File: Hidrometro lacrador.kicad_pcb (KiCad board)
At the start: 2 copper layers, 4 parts, among them U1 ESP32-WROOM-V1

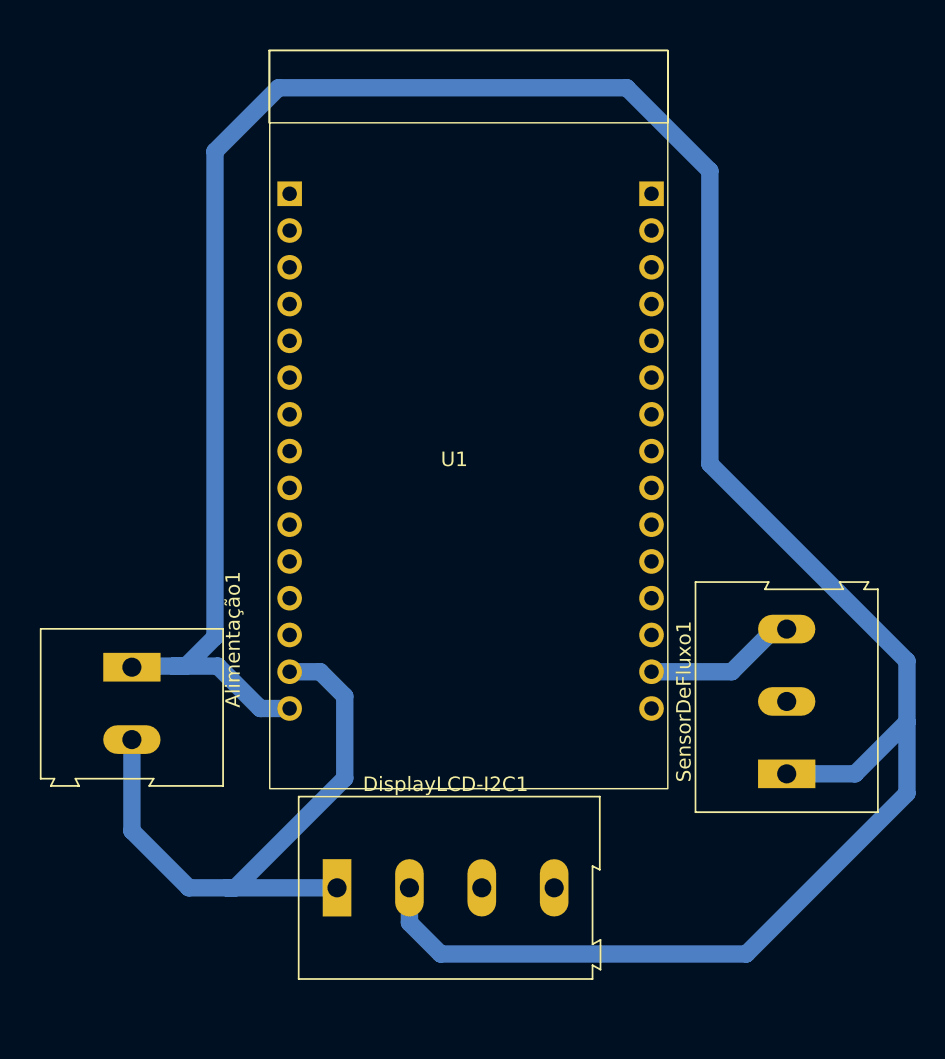
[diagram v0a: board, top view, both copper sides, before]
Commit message: Finalização do circuito e da PCB
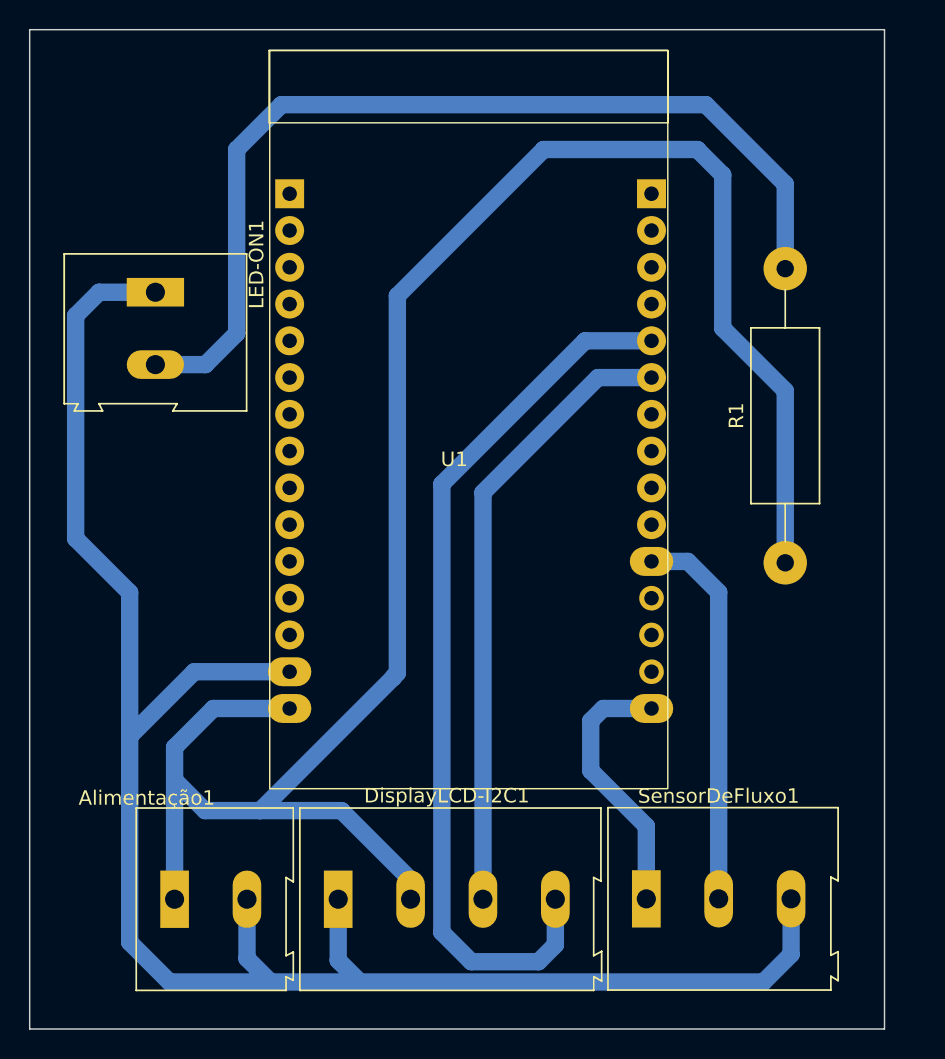
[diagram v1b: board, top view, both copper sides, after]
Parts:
- added LED-ON1: LED, TerminalBlock:TerminalBlock_Altech_AK300-2_P5.00mm, F.Cu at (31.1, 42.4)
- added R1: 330, Resistor_THT:R_Axial_DIN0414_L11.9mm_D4.5mm_P20.32mm_Horizontal, F.Cu at (74.6, 61.1)
- moved Alimentação1 16.3 mm to (32.4, 84.4), turned to 0 degrees
- moved SensorDeFluxo1 13.0 mm to (65.0, 84.3), turned to 0 degrees
- moved DisplayLCD-I2C1 0.79 mm to (43.7, 84.4)
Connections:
- DisplayLCD-I2C1 pad 3: unconnected-(DisplayLCD-I2C1-Pin_3-Pad3) -> I2C_SDA
- DisplayLCD-I2C1 pad 4: unconnected-(DisplayLCD-I2C1-Pin_4-Pad4) -> I2C_SCL
- SensorDeFluxo1 pad 1: +5V -> +3.3V
- SensorDeFluxo1 pad 2: unconnected-(SensorDeFluxo1-Pin_2-Pad2) -> GPIO-04
- U1 pad 20: unconnected-(U1-GPI21/I2C_SDA-Pad20) -> I2C_SCL
- U1 pad 21: unconnected-(U1-GPI19/VSPI_MISO-Pad21) -> I2C_SDA
- U1 pad 26: unconnected-(U1-GPIO04/ADC10-Pad26) -> GPIO-04
- U1 pad 30: unconnected-(U1-3.3V-Pad30) -> +3.3V
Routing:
- net GND: track 54.1 -> 128.1 mm
- net Net-(LED-ON1-A): track 0.00 -> 66.5 mm
- net I2C_SCL: track 0.00 -> 61.9 mm
- net +5V: track 190.3 -> 135.6 mm
- net I2C_SDA: track 0.00 -> 43.0 mm
- net GPIO-04: track 0.00 -> 26.7 mm
- net +3.3V: track 0.00 -> 18.4 mm
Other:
- board outline added: 59.1 x 69 mm
